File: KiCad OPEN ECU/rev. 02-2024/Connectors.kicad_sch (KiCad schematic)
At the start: 3 parts, among them J1 Delphi_Sicma_24, J2 Delphi_Sicma_24

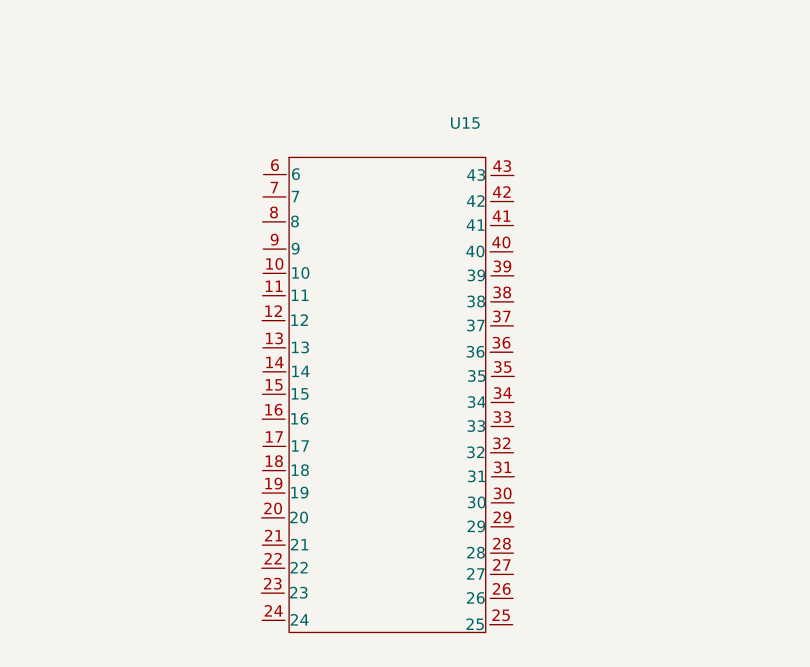
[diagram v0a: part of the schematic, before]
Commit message: update
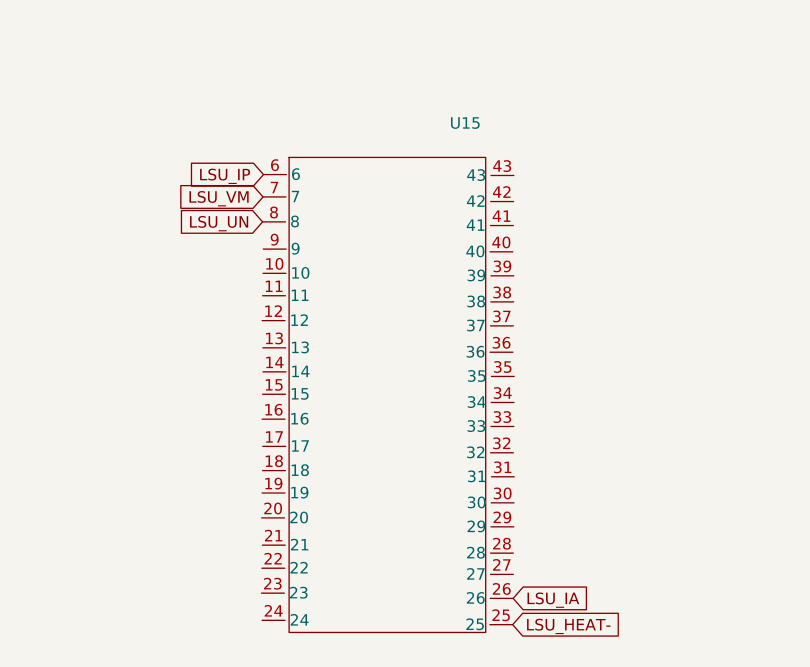
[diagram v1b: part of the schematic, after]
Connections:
- net LSU_HEAT-: now reaches U15.25
- net LSU_IA: now reaches U15.26
- net LSU_IP: now reaches U15.6
- net LSU_VM: now reaches U15.7
- net LSU_UN: now reaches U15.8
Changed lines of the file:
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@@
+    )
+  )
+  (global_label "LSU_HEAT-" (shape input) (at 157.0482 160.147 0) (fields_autoplaced)
+    (effects (font (size 1.27 1.27)) (justify left))
+    (property "Intersheetrefs" "${INTERSHEET_REFS}" (at 170.023 160.147 0)
+      (effects (font (size 1.27 1.27)) (justify left) hide)
     )
   )
@@
     )
   )
+  (global_label "LSU_VM" (shape input) (at 129.3114 112.6236 180) (fields_autoplaced)
+    (effects (font (size 1.27 1.27)) (justify right))
+    (property "Intersheetrefs" "${INTERSHEET_REFS}" (at 119.9047 112.6236 0)
+      (effects (font (size 1.27 1.27)) (justify right) hide)
+    )
+  )
   (global_label "IGN7" (shape input) (at 99.06 81.28 270) (fields_autoplaced)
     (effects (font (size 1.27 1.27)) (justify right))
@@
     )
   )
+  (global_label "LSU_UN" (shape input) (at 129.2606 115.3922 180) (fields_autoplaced)
+    (effects (font (size 1.27 1.27)) (justify right))
+    (property "Intersheetrefs" "${INTERSHEET_REFS}" (at 119.7329 115.3922 0)
+      (effects (font (size 1.27 1.27)) (justify right) hide)
+    )
+  )
   (global_label "IGN1" (shape input) (at 83.82 81.28 270) (fields_autoplaced)
     (effects (font (size 1.27 1.27)) (justify right))
@@
     )
   )
+  (global_label "LSU_IA" (shape input) (at 157.099 157.226 0) (fields_autoplaced)
+    (effects (font (size 1.27 1.27)) (justify left))
+    (property "Intersheetrefs" "${INTERSHEET_REFS}" (at 165.6591 157.226 0)
+      (effects (font (size 1.27 1.27)) (justify left) hide)
+    )
+  )
   (global_label "STEPPER-A2" (shape input) (at 150.622 40.259 0) (fields_autoplaced)
     (effects (font (size 1.27 1.27)) (justify left))
@@
     )
   )
+  (global_label "LSU_IP" (shape input) (at 129.3622 110.1344 180) (fields_autoplaced)
+    (effects (font (size 1.27 1.27)) (justify right))
+    (property "Intersheetrefs" "${INTERSHEET_REFS}" (at 120.6207 110.1344 0)
+      (effects (font (size 1.27 1.27)) (justify right) hide)
+    )
+  )

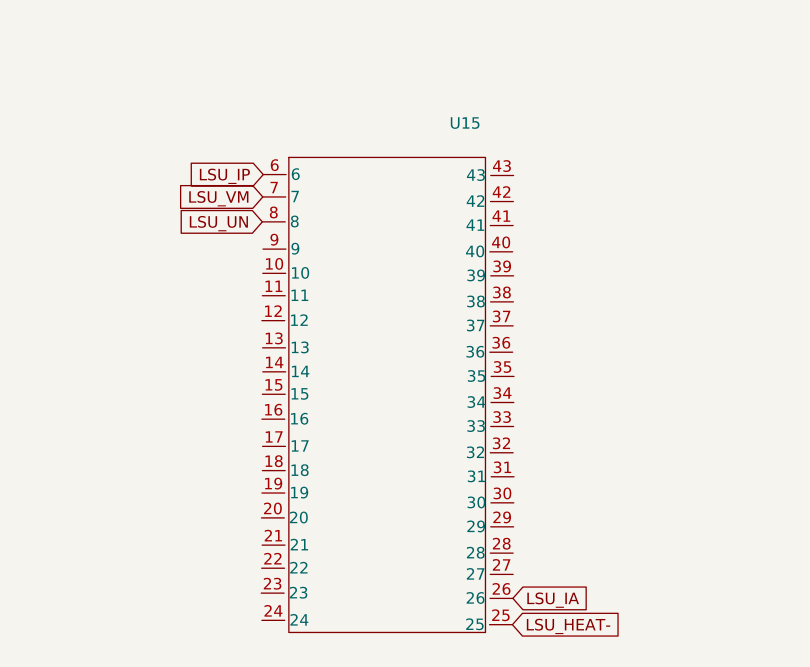
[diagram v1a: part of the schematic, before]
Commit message: update
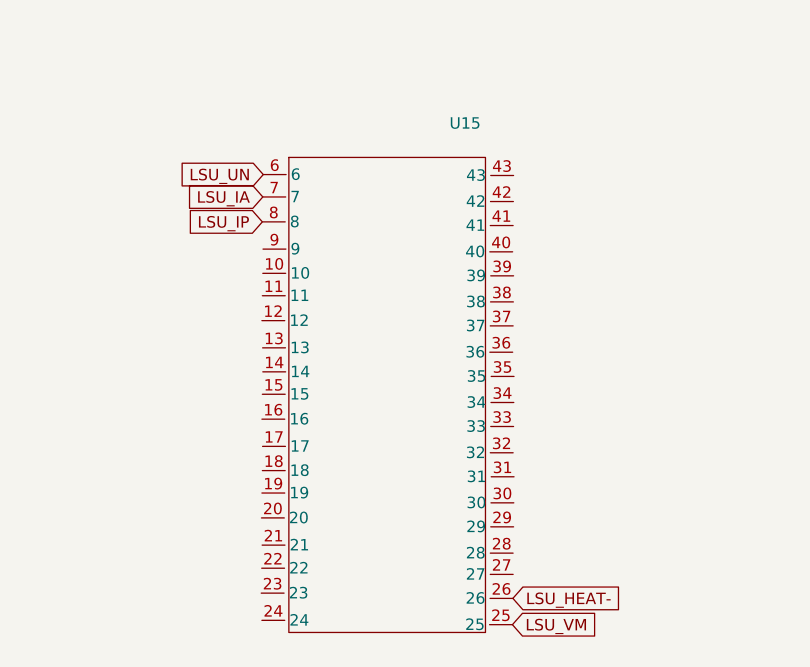
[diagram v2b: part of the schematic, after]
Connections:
- net LSU_HEAT-: now also U15.26; no longer U15.25
- net LSU_IA: now also U15.7; no longer U15.26
- net LSU_IP: now also U15.8; no longer U15.6
- net LSU_UN: now also U15.6; no longer U15.8
- net LSU_VM: now also U15.25; no longer U15.7
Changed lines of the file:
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@@
     )
   )
-  (global_label "LSU_HEAT-" (shape input) (at 157.0482 160.147 0) (fields_autoplaced)
-    (effects (font (size 1.27 1.27)) (justify left))
-    (property "Intersheetrefs" "${INTERSHEET_REFS}" (at 170.023 160.147 0)
+  (global_label "LSU_HEAT-" (shape input) (at 157.099 157.226 0) (fields_autoplaced)
+    (effects (font (size 1.27 1.27)) (justify left))
+    (property "Intersheetrefs" "${INTERSHEET_REFS}" (at 170.0738 157.226 0)
       (effects (font (size 1.27 1.27)) (justify left) hide)
     )
@@
     )
   )
-  (global_label "LSU_VM" (shape input) (at 129.3114 112.6236 180) (fields_autoplaced)
-    (effects (font (size 1.27 1.27)) (justify right))
-    (property "Intersheetrefs" "${INTERSHEET_REFS}" (at 119.9047 112.6236 0)
-      (effects (font (size 1.27 1.27)) (justify right) hide)
+  (global_label "LSU_VM" (shape input) (at 157.0482 160.147 0) (fields_autoplaced)
+    (effects (font (size 1.27 1.27)) (justify left))
+    (property "Intersheetrefs" "${INTERSHEET_REFS}" (at 166.4549 160.147 0)
+      (effects (font (size 1.27 1.27)) (justify left) hide)
     )
   )
@@
     )
   )
-  (global_label "LSU_UN" (shape input) (at 129.2606 115.3922 180) (fields_autoplaced)
-    (effects (font (size 1.27 1.27)) (justify right))
-    (property "Intersheetrefs" "${INTERSHEET_REFS}" (at 119.7329 115.3922 0)
+  (global_label "LSU_UN" (shape input) (at 129.3622 110.1344 180) (fields_autoplaced)
+    (effects (font (size 1.27 1.27)) (justify right))
+    (property "Intersheetrefs" "${INTERSHEET_REFS}" (at 119.8345 110.1344 0)
       (effects (font (size 1.27 1.27)) (justify right) hide)
     )
@@
     )
   )
-  (global_label "LSU_IA" (shape input) (at 157.099 157.226 0) (fields_autoplaced)
-    (effects (font (size 1.27 1.27)) (justify left))
-    (property "Intersheetrefs" "${INTERSHEET_REFS}" (at 165.6591 157.226 0)
-      (effects (font (size 1.27 1.27)) (justify left) hide)
+  (global_label "LSU_IA" (shape input) (at 129.3114 112.6236 180) (fields_autoplaced)
+    (effects (font (size 1.27 1.27)) (justify right))
+    (property "Intersheetrefs" "${INTERSHEET_REFS}" (at 120.7513 112.6236 0)
+      (effects (font (size 1.27 1.27)) (justify right) hide)
     )
   )
@@
     )
   )
-  (global_label "LSU_IP" (shape input) (at 129.3622 110.1344 180) (fields_autoplaced)
-    (effects (font (size 1.27 1.27)) (justify right))
-    (property "Intersheetrefs" "${INTERSHEET_REFS}" (at 120.6207 110.1344 0)
-      (effects (font (size 1.27 1.27)) (justify right) hide)
-    )
+  (global_label "LSU_IP" (shape input) (at 129.2606 115.3922 180) (fields_autoplaced)
+    (effects (font (size 1.27 1.27)) (justify right))
+    (property "Intersheetrefs" "${INTERSHEET_REFS}" (at 120.5191 115.3922 0)
+      (effects (font (size 1.27 1.27)) (justify right) hide)
+    )
